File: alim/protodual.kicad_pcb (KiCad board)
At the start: 2 copper layers, 99.6 x 87.4 mm, 72 parts, among them P1 BATT_IN, P2 ALIM_L1, P3 ALIM_PW1, P4 ARU, P5 SW_LOGIC, Q1 Q_NMOS_DGS, Q2 Q_NMOS_DGS, Q3 Q_NMOS_DGS, Q4 Q_NMOS_DGS, Q5 Q_PMOS_GDS, Q6 Q_PMOS_GDS, U1 LM25119, U2 TRACO3.3, U3 TRACO5, U4 TRACO15

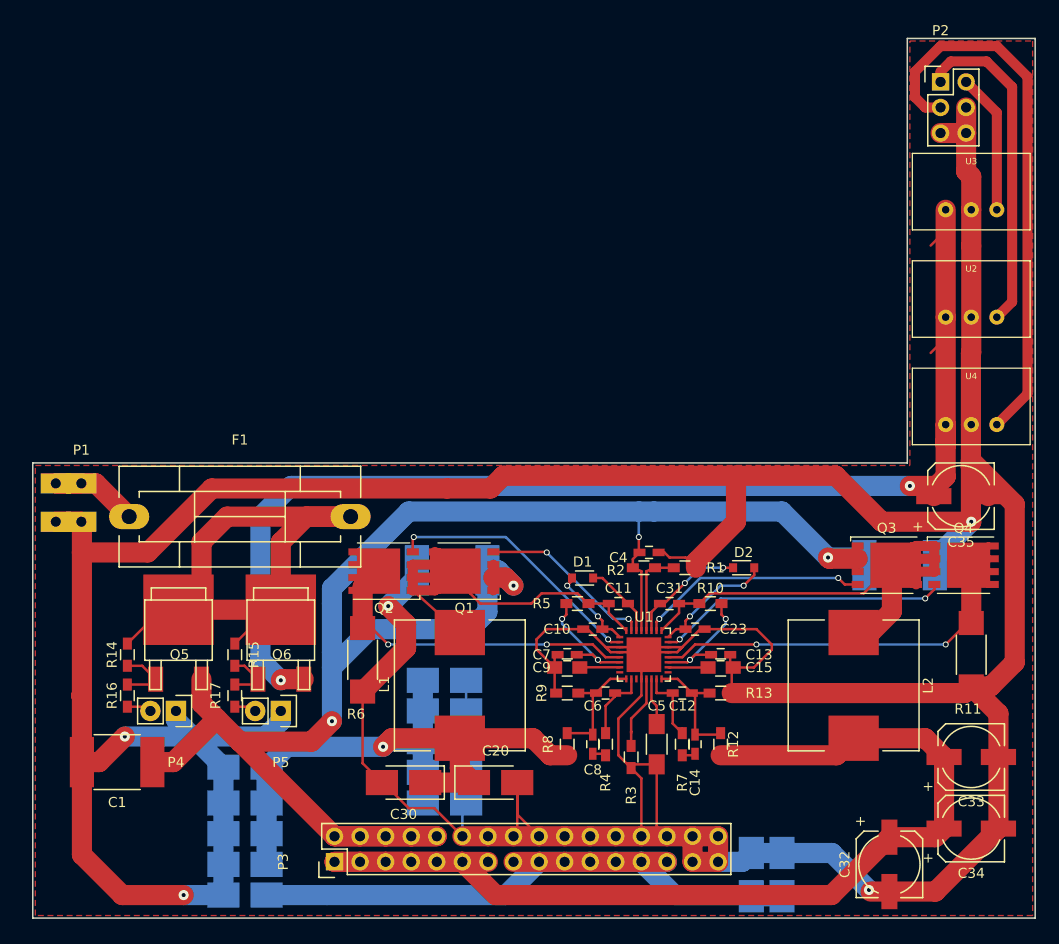
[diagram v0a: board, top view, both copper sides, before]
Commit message: ALim a grosse piste
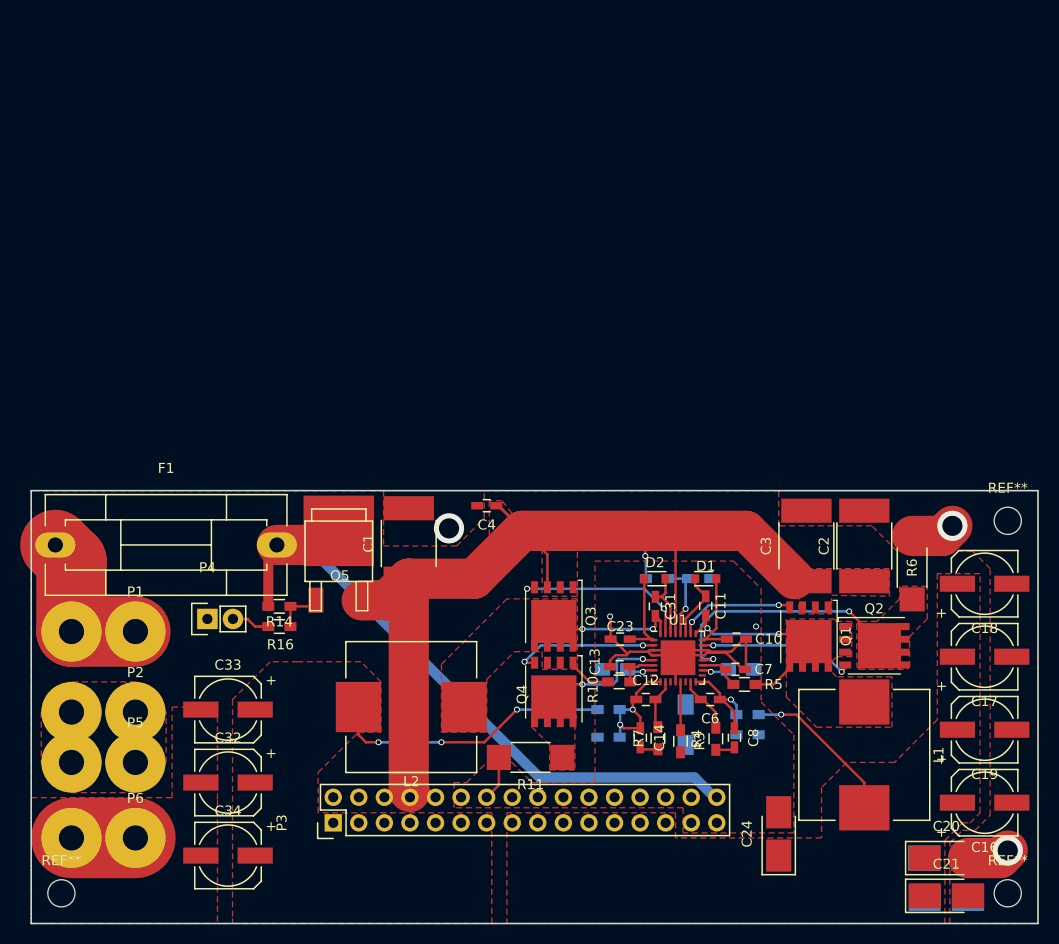
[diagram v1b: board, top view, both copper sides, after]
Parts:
- removed C26, C27, C28, C29, C30: 100uF, Capacitors_Tantalum_SMD:Tantalum_Case-B_EIA-3528-21_Hand
- removed C35: 22uF/50V, Capacitors_SMD:c_elec_6.3x5.3
- removed Q6: Q_PMOS_GDS, TO_SOT_Packages_SMD:SOT-428
- removed R15: 10k, Resistors_SMD:R_0603_HandSoldering
- removed R17: 8k, Resistors_SMD:R_0603_HandSoldering
- removed U2: TRACO3.3, kicad-library:TRACO-TSR-1-DC-DC
- removed U3: TRACO5, kicad-library:TRACO-TSR-1-DC-DC
- removed U4: TRACO15, kicad-library:TRACO-TSR-1-DC-DC
- added P6: BAT2-, kicad-library:WireConnection_2.50mm, F.Cu at (99.3, 132.5)
- added REF**: MountingHole_2.7mm_M2.5_ISO14580, Mounting_Holes:MountingHole_2.7mm_M2.5_ISO14580, F.Cu at (186.0, 101.0)
- added REF**: MountingHole_2.7mm_M2.5_ISO14580, Mounting_Holes:MountingHole_2.7mm_M2.5_ISO14580, F.Cu at (186.0, 138.0)
- added REF**: MountingHole_2.7mm_M2.5_ISO14580, Mounting_Holes:MountingHole_2.7mm_M2.5_ISO14580, F.Cu at (92.0, 138.0)
- C15, C5, C9, R1, R12, R13, R2, R8, R9: moved to B.Cu
- C16, C17, C18, C19: value 100uF -> 270uF; footprint Capacitors_Tantalum_SMD:Tantalum_Case-B_EIA-3528-21_Hand -> Capacitors_SMD:c_elec_6.3x7.7; moved to F.Cu
- C2, C21, C24, C3: moved to F.Cu
- P1: value BATT_IN -> BAT1+; footprint kicad-library:BATT_SOLDERPAD -> kicad-library:WireConnection_2.50mm
- P2: value ALIM_L1 -> BAT1-; footprint Pin_Headers:Pin_Header_Straight_2x03 -> kicad-library:WireConnection_2.50mm
- P5: value SW_LOGIC -> BAT2+; footprint Socket_Strips:Socket_Strip_Straight_1x02 -> kicad-library:WireConnection_2.50mm
- moved P2 101.6 mm to (99.3, 120.0), turned to 180 degrees
- moved C18 76.6 mm to (183.7, 107.2), turned to 0 degrees
- moved C17 75.5 mm to (183.7, 114.5), turned to 0 degrees
- moved C16 74.0 mm to (183.7, 129.0), turned to 0 degrees
- moved C33 74.0 mm to (108.5, 119.8), turned to 180 degrees
- moved C34 73.9 mm to (108.5, 134.2), turned to 180 degrees
- moved C32 66.2 mm to (108.5, 127.0), turned to 180 degrees
- moved R6 55.3 mm to (176.5, 105.7), turned to 90 degrees
- moved C19 53.8 mm to (183.7, 121.8)
- moved C24 53.1 mm to (163.2, 132.1), turned to 90 degrees
- moved C21 52.2 mm to (179.9, 138.2)
- moved C22 50.1 mm to (179.8, 134.5)
- moved Q2 49.3 mm to (172.8, 113.4), turned to 0 degrees
- moved C20 45.4 mm to (179.9, 134.5)
- moved R11 44.9 mm to (138.6, 124.5), turned to 180 degrees
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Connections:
- P1 pad 1: GND -> Net-(F1-Pad1)
- P2 pad 1: VL33 -> Net-(P2-Pad1)
- P3 pad 32: GND -> VBATT
- P5 pad 1: GND -> Net-(P2-Pad1)
- U1 pad 1: Net-(C10-Pad1) -> Net-(C23-Pad1)
- U1 pad 10: Net-(C6-Pad2) -> Net-(C12-Pad2)
- U1 pad 15: Net-(C12-Pad2) -> Net-(C6-Pad2)
- U1 pad 16: FBCK2 -> FBCK1
- U1 pad 18: Net-(C15-Pad1) -> Net-(C9-Pad1)
- U1 pad 19: Net-(C13-Pad1) -> Net-(C7-Pad1)
- U1 pad 2: Net-(Q2-Pad2) -> Net-(Q4-Pad2)
- U1 pad 20: Net-(Q4-Pad3) -> Net-(Q2-Pad3)
- U1 pad 23: Net-(Q4-Pad2) -> Net-(Q2-Pad2)
- U1 pad 24: Net-(C23-Pad1) -> Net-(C10-Pad1)
- U1 pad 25: Net-(C31-Pad2) -> Net-(C11-Pad1)
- U1 pad 26: Net-(Q3-Pad2) -> Net-(Q1-Pad2)
- U1 pad 27: Net-(C31-Pad1) -> Net-(C11-Pad2)
- U1 pad 30: Net-(C11-Pad2) -> Net-(C31-Pad1)
- U1 pad 31: Net-(Q1-Pad2) -> Net-(Q3-Pad2)
- U1 pad 32: Net-(C11-Pad1) -> Net-(C31-Pad2)
- U1 pad 5: Net-(Q2-Pad3) -> Net-(Q4-Pad3)
- U1 pad 6: Net-(C7-Pad1) -> Net-(C13-Pad1)
- U1 pad 7: Net-(C9-Pad1) -> Net-(C15-Pad1)
- U1 pad 9: FBCK1 -> FBCK2
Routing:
- net GND: track 659.1 -> 52.2 mm
- net Net-(C35-Pad1): track 127.7 -> 0.00 mm, vias 2 -> 0
- net VOUT1: track 139.3 -> 15.8 mm
- net VOUT2: track 110.7 -> 28.2 mm, vias 0 -> 3
- net +BATT: track 178.7 -> 97.8 mm, vias 4 -> 1
- net VL15: track 54.8 -> 0.00 mm
- net Net-(C31-Pad2): track 61.9 -> 16.7 mm, vias 0 -> 2
- net VL33: track 33.6 -> 0.00 mm
- net Net-(Q4-Pad3): track 37.4 -> 11.2 mm
- net Net-(C11-Pad1): track 41.5 -> 19.8 mm, vias 0 -> 2
- net Net-(Q4-Pad2): track 29.1 -> 14.6 mm
- net VL5: track 14.0 -> 0.00 mm
- net Net-(Q2-Pad3): track 36.0 -> 24.1 mm
- net Net-(Q2-Pad2): track 26.3 -> 15.8 mm
- net Net-(C13-Pad1): track 12.1 -> 4.05 mm, vias 2 -> 0
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- added copper zone on F.Cu, net +BATT
- added copper zone on B.Cu, net GND
- added copper zone on F.Cu, net Net-(C11-Pad1)
- added copper zone on F.Cu, net Net-(C31-Pad2)
- added copper zone on F.Cu, net Net-(P2-Pad1)
- added copper zone on F.Cu, net Net-(Q2-Pad3)
- added copper zone on F.Cu, net Net-(Q4-Pad3)
- added copper zone on F.Cu, net VOUT1
- added copper zone on F.Cu, net VOUT2
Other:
- board size 99.6 x 87.4 mm -> 100 x 43 mm
- net class Power: trace_width 2 -> 4; via_dia 1 -> 3; via_drill 0.4 -> 2
- net class VBatt added: clearance 0.8, trace_width 1, via_dia 0.8, via_drill 0.5
